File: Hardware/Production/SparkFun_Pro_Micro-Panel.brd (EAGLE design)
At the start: 104.6 x 128.3 mm, 1563 parts, among them J1 Qwiic, J13 Qwiic, J17 Qwiic, J2 Qwiic, J21 Qwiic, J25 Qwiic, J29 Qwiic, J33 Qwiic, J37 Qwiic, J41 Qwiic, J45 Qwiic, J49 Qwiic, J53 Qwiic, J57 Qwiic, J9 Qwiic, U1 3.3V, U10 3.3V, U11 ATmega32U4, U12 3.3V, U13 ATmega32U4, U14 3.3V, U15 ATmega32U4, U16 3.3V, U17 ATmega32U4, U18 3.3V, U19 ATmega32U4, U2 ATmega32U4, U20 3.3V, U21 ATmega32U4, U22 3.3V, U23 ATmega32U4, U24 3.3V, U25 ATmega32U4, U26 3.3V, U27 ATmega32U4, U28 3.3V, U29 ATmega32U4, U3 ATmega32U4, U30 3.3V, U4 3.3V, U5 ATmega32U4, U6 3.3V, U7 ATmega32U4, U8 3.3V, U9 ATmega32U4, Y1 32MHz, Y10 32MHz, Y11 32MHz, Y12 32MHz, Y13 32MHz, Y14 32MHz, Y15 32MHz, Y2 32MHz, Y3 32MHz, Y4 32MHz, Y5 32MHz, Y6 32MHz, Y7 32MHz, Y8 32MHz, Y9 32MHz

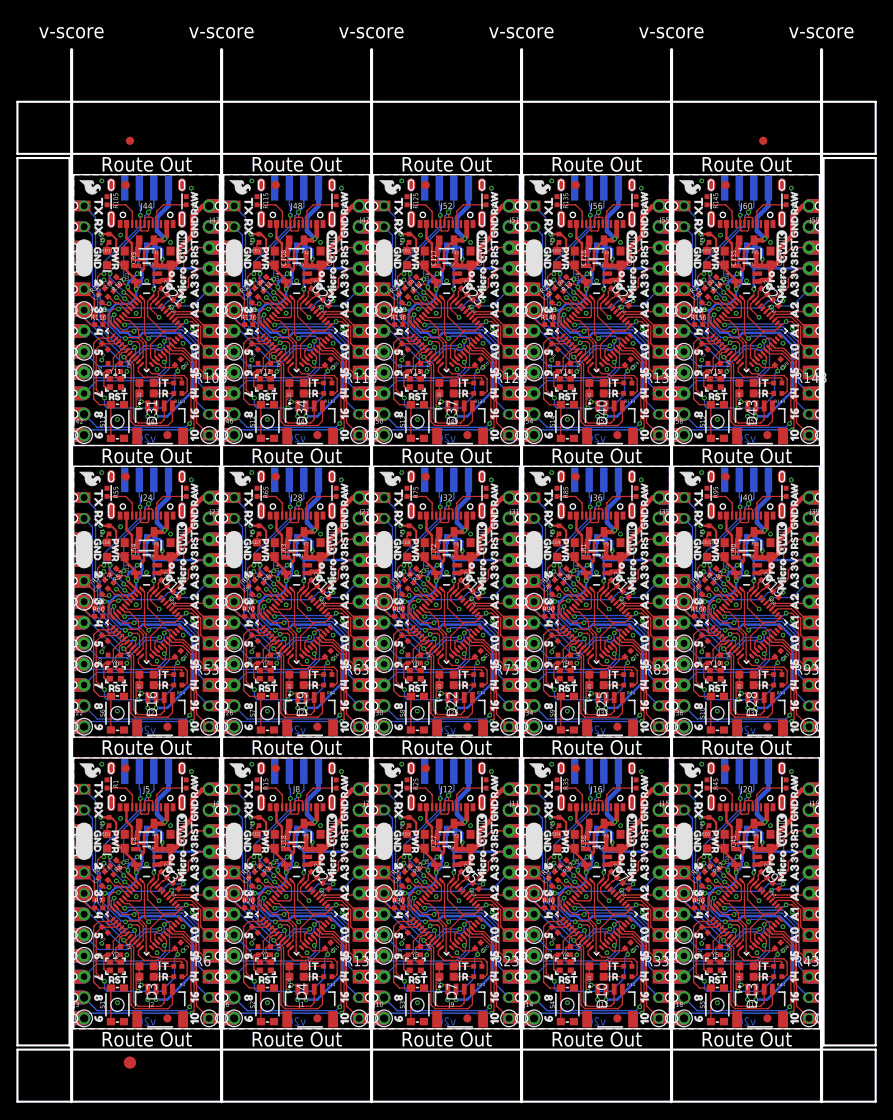
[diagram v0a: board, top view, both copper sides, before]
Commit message: Adding production panel, pro micro FP test brd, and castellated test lbr.
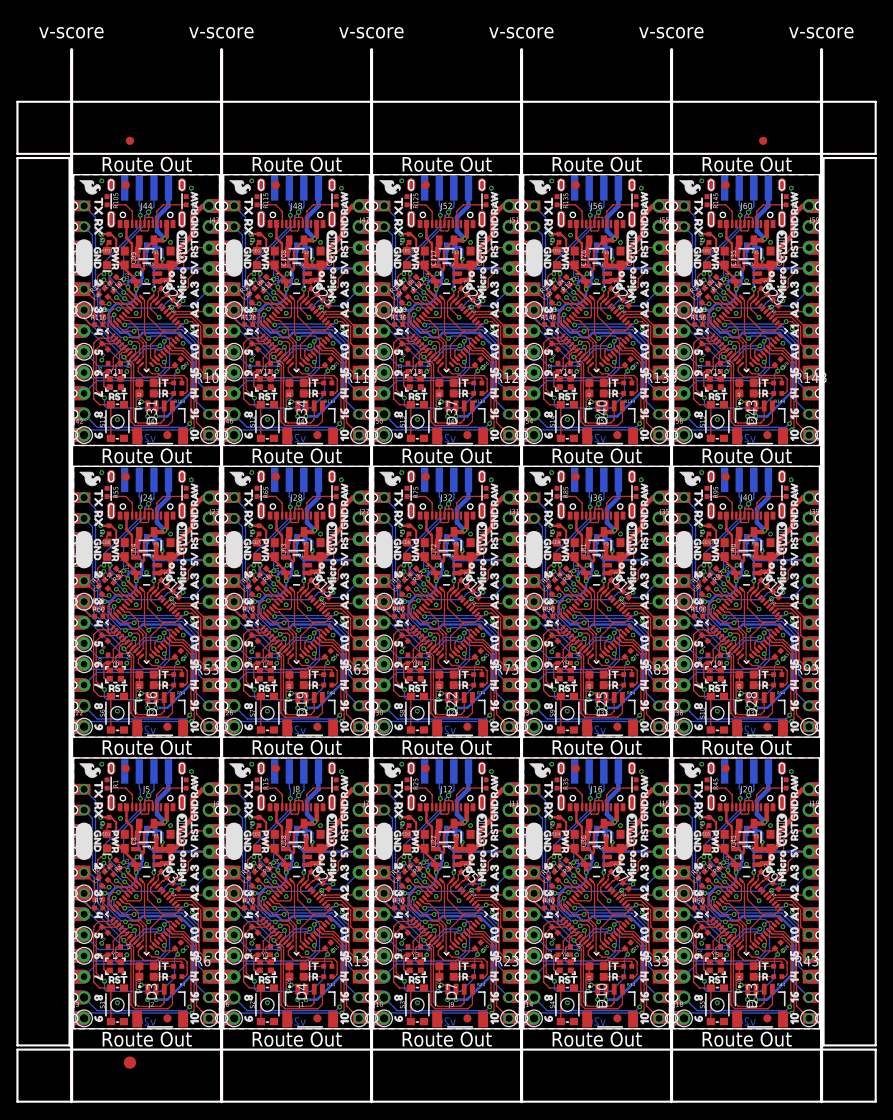
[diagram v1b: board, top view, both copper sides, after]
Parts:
- U$100, U$164, U$228, U$292, U$356, U$420, U$484, U$548, U$612, U$676, U$740, U$804, U$868, U$932: device buzzard_labels (18):3V39 -> buzzard_labels (15):A29
- U$101, U$165, U$229, U$293, U$357, U$421, U$485, U$549, U$613, U$677, U$741, U$805, U$869, U$933: device buzzard_labels (15):A310 -> buzzard_labels (15):A18
- U$102, U$166, U$230, U$294, U$358, U$422, U$486, U$550, U$614, U$678, U$742, U$806, U$870, U$934: device buzzard_labels (15):A29 -> buzzard_labels (15):A07
- U$103, U$167, U$231, U$295, U$359, U$423, U$487, U$551, U$615, U$679, U$743, U$807, U$871, U$935: device buzzard_labels (15):A18 -> buzzard_labels (15):156
- U$104, U$168, U$232, U$296, U$360, U$424, U$488, U$552, U$616, U$680, U$744, U$808, U$872, U$936: device buzzard_labels (15):A07 -> buzzard_labels (15):145
- U$105, U$169, U$233, U$297, U$361, U$425, U$489, U$553, U$617, U$681, U$745, U$809, U$873, U$937: device buzzard_labels (15):156 -> buzzard_labels (15):164
- U$106, U$170, U$234, U$298, U$362, U$426, U$490, U$554, U$618, U$682, U$746, U$810, U$874, U$938: device buzzard_labels (15):145 -> buzzard_labels (14):104
- U$107, U$171, U$235, U$299, U$363, U$427, U$491, U$555, U$619, U$683, U$747, U$811, U$875, U$939: device buzzard_labels (15):164 -> buzzard_labels (15):911
- U$108, U$172, U$236, U$300, U$364, U$428, U$492, U$556, U$620, U$684, U$748, U$812, U$876, U$940: device buzzard_labels (14):104 -> buzzard_labels (15):812
- U$109, U$173, U$237, U$301, U$365, U$429, U$493, U$557, U$621, U$685, U$749, U$813, U$877, U$941: device buzzard_labels (15):911 -> buzzard_labels (15):713
- U$110, U$174, U$238, U$302, U$366, U$430, U$494, U$558, U$622, U$686, U$750, U$814, U$878, U$942: device buzzard_labels (15):812 -> buzzard_labels (15):614
- U$111, U$175, U$239, U$303, U$367, U$431, U$495, U$559, U$623, U$687, U$751, U$815, U$879, U$943: device buzzard_labels (15):713 -> buzzard_labels (15):515
- U$112, U$176, U$240, U$304, U$368, U$432, U$496, U$560, U$624, U$688, U$752, U$816, U$880, U$944: device buzzard_labels (15):614 -> buzzard_labels (13):45
- U$113, U$177, U$241, U$305, U$369, U$433, U$497, U$561, U$625, U$689, U$753, U$817, U$881, U$945: device buzzard_labels (15):515 -> buzzard_labels (15):317
- U$114, U$178, U$242, U$306, U$370, U$434, U$498, U$562, U$626, U$690, U$754, U$818, U$882, U$946: device buzzard_labels (13):45 -> buzzard_labels (15):218
- U$115, U$179, U$243, U$307, U$371, U$435, U$499, U$563, U$627, U$691, U$755, U$819, U$883, U$947: device buzzard_labels (15):317 -> buzzard_labels (16):GND4
- U$116, U$180, U$244, U$308, U$372, U$436, U$500, U$564, U$628, U$692, U$756, U$820, U$884, U$948: device buzzard_labels (15):218 -> buzzard_labels (15):RX20
- U$117, U$181, U$245, U$309, U$373, U$437, U$501, U$565, U$629, U$693, U$757, U$821, U$885, U$949: device buzzard_labels (16):GND4 -> buzzard_labels (13):TX2
- U$118, U$182, U$246, U$310, U$374, U$438, U$502, U$566, U$630, U$694, U$758, U$822, U$886, U$950: device buzzard_labels (15):RX20 -> buzzard_labels (17):GND4
- U$119, U$183, U$247, U$311, U$375, U$439, U$503, U$567, U$631, U$695, U$759, U$823, U$887, U$951: device buzzard_labels (13):TX2 -> buzzard_labels (18):3V39
- U$120, U$184, U$248, U$312, U$376, U$440, U$504, U$568, U$632, U$696, U$760, U$824, U$888, U$952: device buzzard_labels (17):GND4 -> buzzard_labels (13):G1
- U$121, U$185, U$249, U$313, U$377, U$441, U$505, U$569, U$633, U$697, U$761, U$825, U$889, U$953: device buzzard_labels (18):3V39 -> buzzard_labels (13):V0
- U$122, U$186, U$250, U$314, U$378, U$442, U$506, U$570, U$634, U$698, U$762, U$826, U$890, U$954: device buzzard_labels (13):G1 -> buzzard_labels (14):D#3
- U$123, U$187, U$251, U$315, U$379, U$443, U$507, U$571, U$635, U$699, U$763, U$827, U$891, U$955: device buzzard_labels (13):V0 -> buzzard_labels (14):D#4
- U$124, U$188, U$252, U$316, U$380, U$444, U$508, U$572, U$636, U$700, U$764, U$828, U$892, U$956: device buzzard_labels (14):D#3 -> buzzard_labels (10):PWR0
- U$125, U$189, U$253, U$317, U$381, U$445, U$509, U$573, U$637, U$701, U$765, U$829, U$893, U$957: device buzzard_labels (14):D#4 -> buzzard_labels (10):5V1
- U$126, U$190, U$254, U$318, U$382, U$446, U$510, U$574, U$638, U$702, U$766, U$830, U$894, U$958: device buzzard_labels (10):PWR0 -> buzzard_labels (11):VCC1
- U$128, U$192, U$256, U$320, U$384, U$448, U$512, U$576, U$640, U$704, U$768, U$832, U$896, U$960: device buzzard_labels (11):VCC1 -> buzzard_labels (10):5V1
- U$15: device buzzard_labels (18):3V39 -> buzzard_labels (10):5V1
- U$163, U$227, U$291, U$355, U$419, U$483, U$547, U$611, U$675, U$739, U$803, U$867, U$931, U$99: device buzzard_labels (18):3V39 -> buzzard_labels (15):A310
- U$33: value (none) -> OSHW-LOGOMINI; device buzzard_labels (18):3V39 -> SparkFun-Aesthetics:OSHW-LOGO-MINI
- U$65: value OSHW-LOGOMINI -> (none); device SparkFun-Aesthetics:OSHW-LOGO-MINI -> buzzard_labels (10):5V1
- moved U$33 23.2 mm to (34.5, 31.5), flipped to the bottom, turned to 0 degrees
- moved U$65 22.9 mm to (14.7, 20.1), flipped to the top, turned to 90 degrees
- moved U$940 12.8 mm to (77.1, 74.9)
- moved U$300 12.8 mm to (77.1, 3.81)
- moved U$620 12.8 mm to (77.1, 39.4)
- moved U$684 12.8 mm to (3.94, 74.9)
- moved U$364 12.8 mm to (3.94, 39.4)
- moved U$748 12.8 mm to (22.2, 74.9)
- moved U$812 12.8 mm to (40.5, 74.9)
- moved U$108 12.8 mm to (22.2, 3.81)
- moved U$172 12.8 mm to (40.5, 3.81)
- moved U$428 12.8 mm to (22.2, 39.4)
- moved U$492 12.8 mm to (40.5, 39.4)
- moved U$876 12.8 mm to (58.8, 74.9)
- moved U$236 12.8 mm to (58.8, 3.81)
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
